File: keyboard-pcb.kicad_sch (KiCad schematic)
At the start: 16 parts, among them J1 USB_C_Receptacle_USB2.0_14P, U1 STM32F072CBTx, U2 XC6206PxxxMR

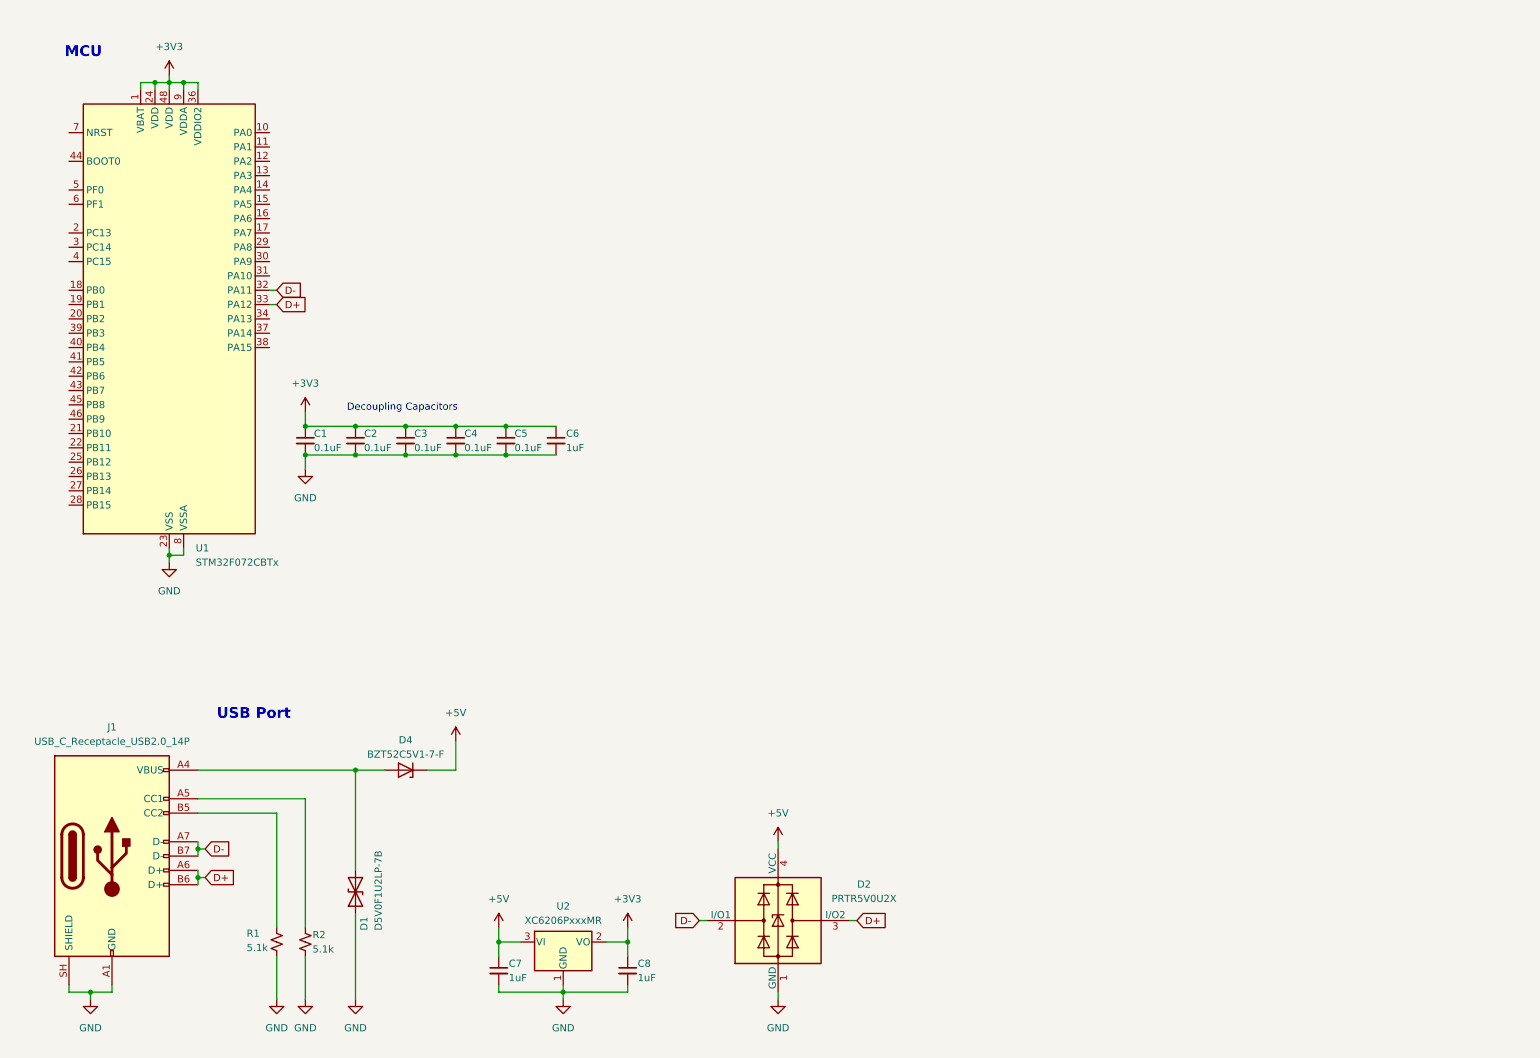
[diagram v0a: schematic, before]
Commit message: finished rest of the schematic
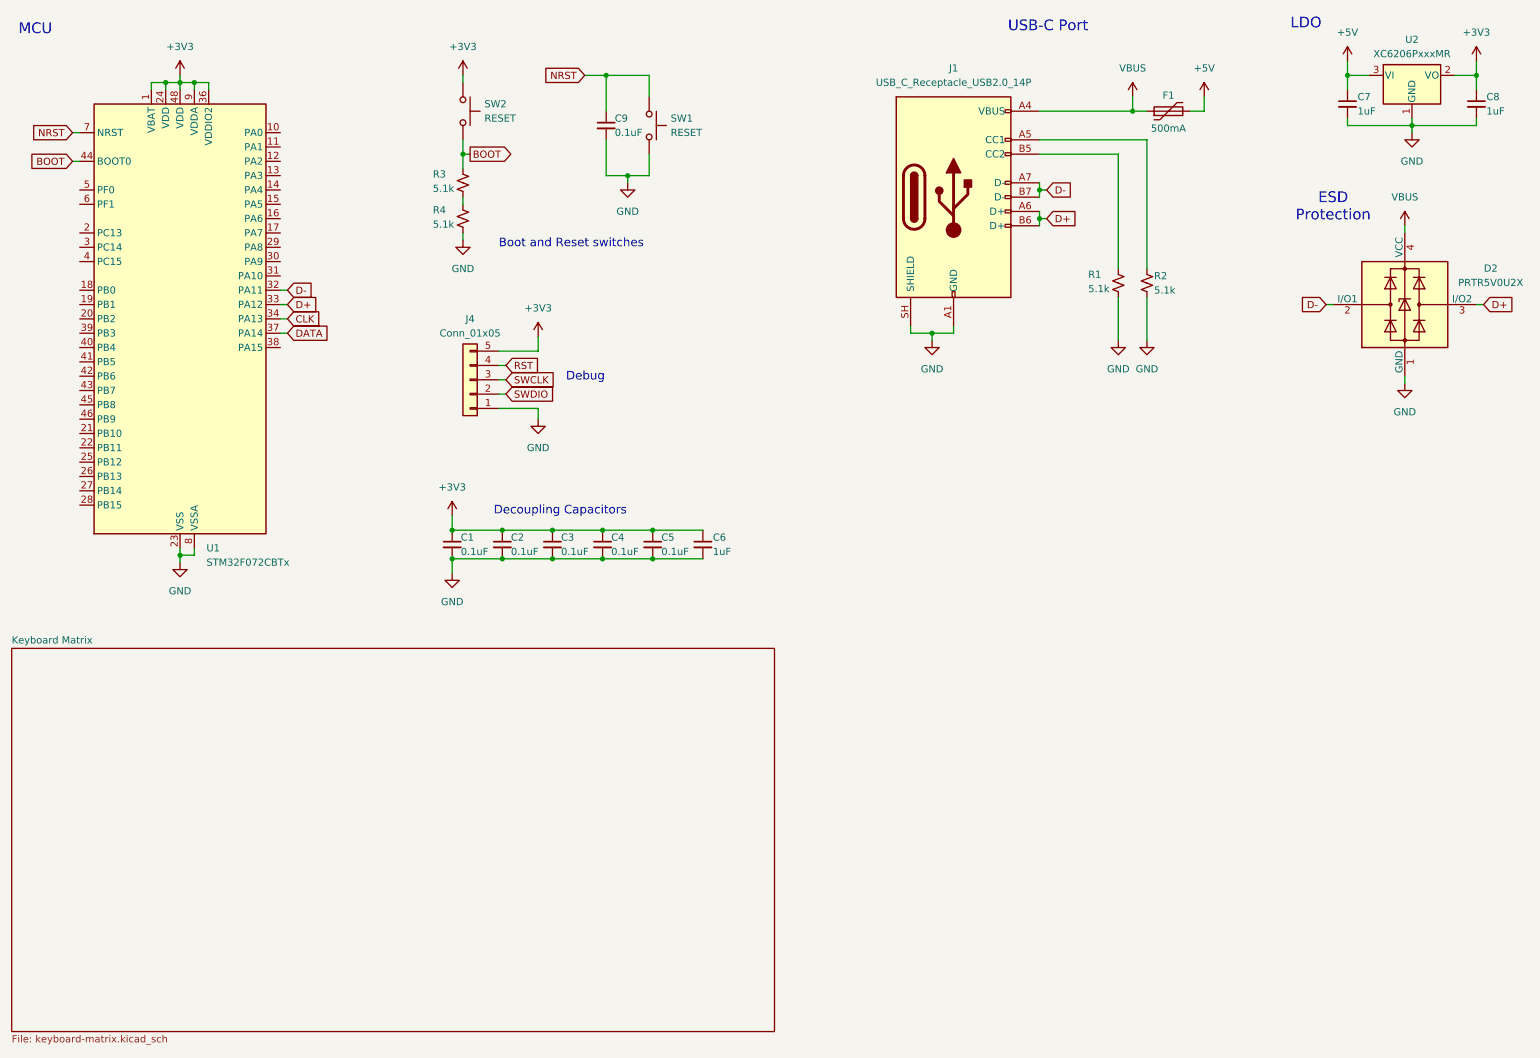
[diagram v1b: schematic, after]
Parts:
- removed D1: D5V0F1U2LP-7B, Diode_SMD:D_0402_1005Metric_Pad0.77x0.64mm_HandSolder, symbol Device:D_TVS
- removed D4: BZT52C5V1-7-F, Diode_SMD:D_SOD-123, symbol Device:D_Zener
- added C9: 0.1uF, symbol Device:C_Small
- added F1: 500mA, symbol Device:Polyfuse
- added J4: Conn_01x05, symbol Connector_Generic:Conn_01x05
- added R3, R4: 5.1k, symbol Device:R_Small_US
- added SW1, SW2: RESET, symbol Switch:SW_Push
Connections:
- net +3V3: now also J4.5 (Pin_5), SW2.1
- net +5V: now also F1.2; no longer D2.4 (VCC)
- net GND: now also C9.2, J4.1 (Pin_1), R4.1, SW1.2
- net VBUS: now reaches J1.A4 (VBUS), J1.A9 (VBUS), J1.B4 (VBUS), J1.B9 (VBUS)
- net VBUS: now also D2.4 (VCC), F1.1
- net CLK: now reaches U1.34 (PA13)
- net DATA: now reaches U1.37 (PA14)
- net BOOT: now reaches U1.44 (BOOT0)
- net BOOT: now also R3.2, SW2.2
- net NRST: now reaches U1.7 (NRST)
- net NRST: now also C9.1, SW1.1
- new net: R3.1, R4.2
- new net RST: J4.4 (Pin_4)
- new net SWCLK: J4.3 (Pin_3)
- new net SWDIO: J4.2 (Pin_2)
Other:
- added sheet Keyboard Matrix (keyboard-matrix.kicad_sch)
- note added: "Boot and Reset switches"
- note added: "Debug"
- note added: "ESD Protection"
- note added: "LDO"
- note added: "USB-C Port"
- note removed: "USB Port"
- title: (none) -> AwesomeKey
- moved on the sheet: C1, C2, C3, C4, C5, C6, C7, C8, D2, J1, R1, R2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
